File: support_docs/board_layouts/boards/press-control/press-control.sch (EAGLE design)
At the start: 19 parts

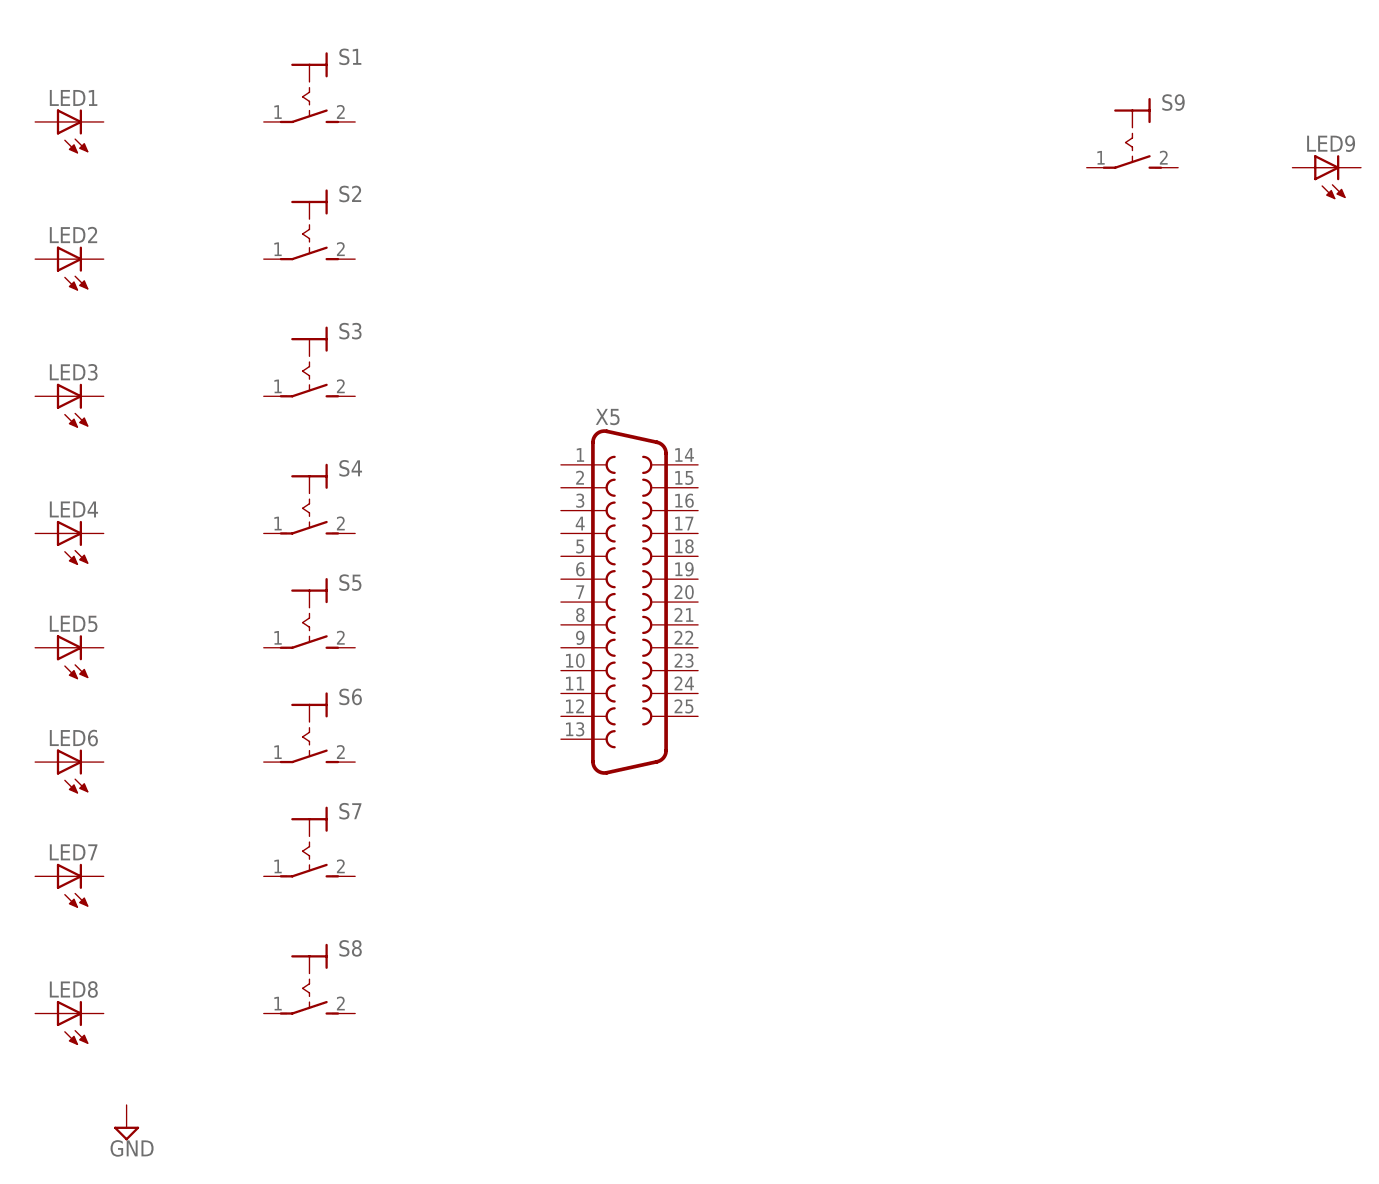
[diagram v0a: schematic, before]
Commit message: new board design
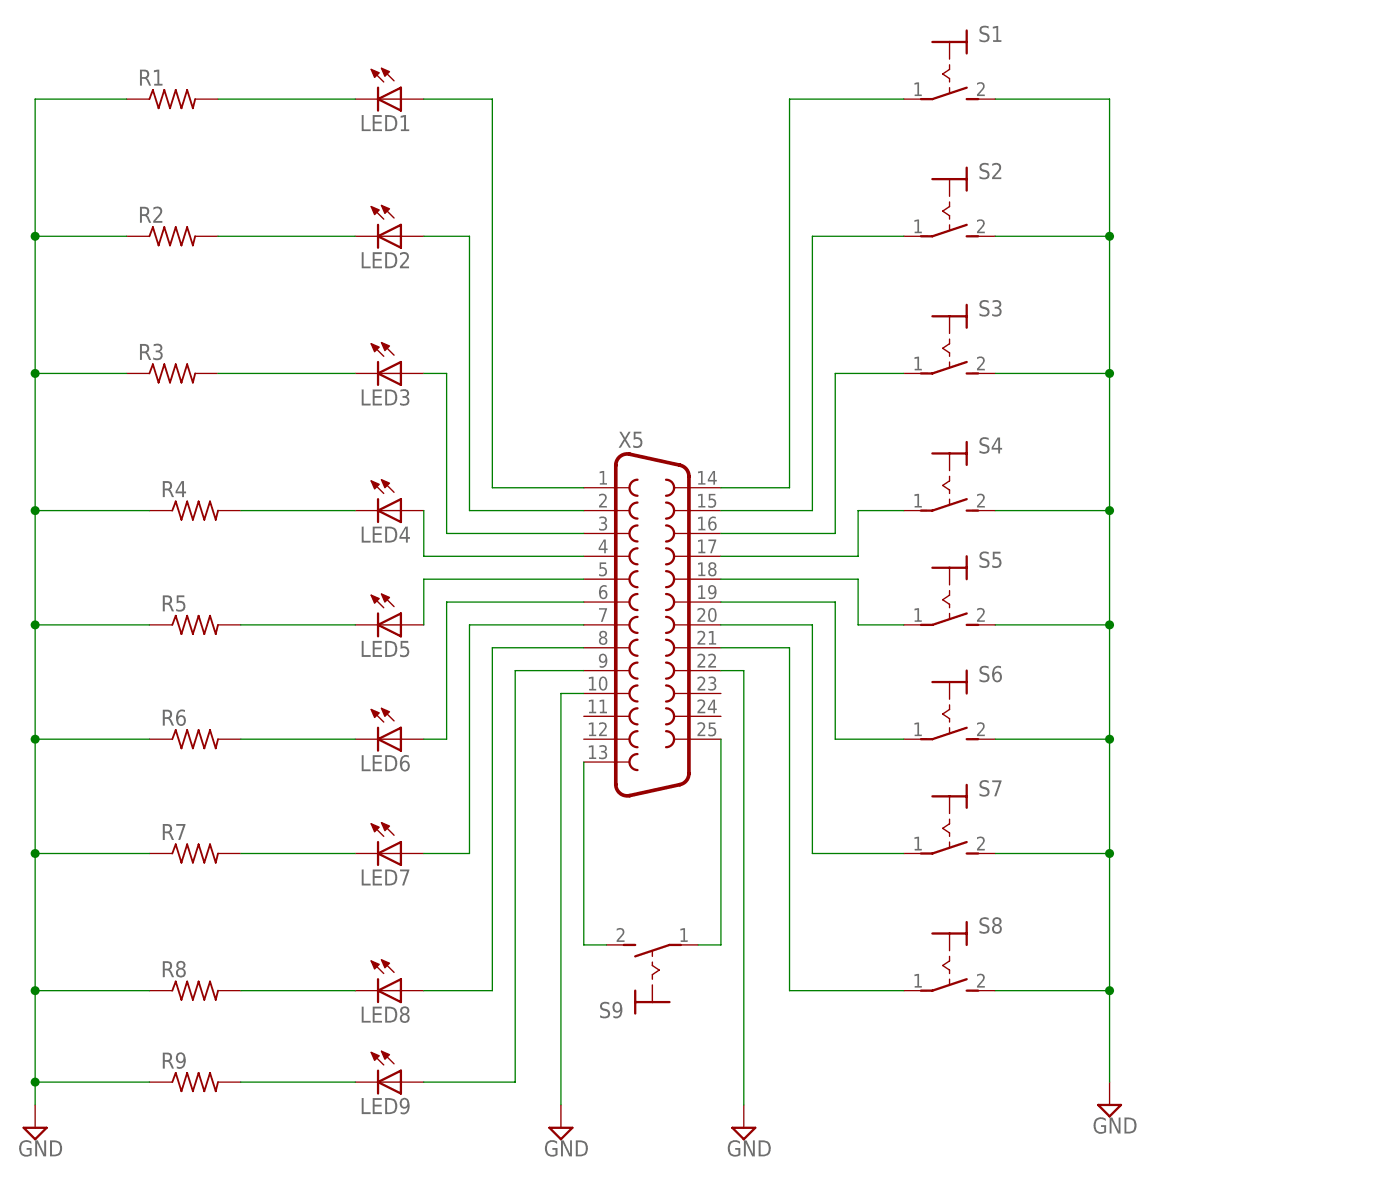
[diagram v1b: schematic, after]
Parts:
- added R1, R2, R3, R4, R5, R6, R7, R8, R9: (no value), resistor:R-US_0207/10
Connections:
- new net GND: R1.1, R2.1, R3.1, R4.1, R5.1, R6.1, R7.1, R8.1, R9.1, S1.S, S2.S, S3.S, S4.S, S5.S, S6.S, S7.S, S8.S, X5.10, X5.22
- new net N$1: LED1.C, R1.2
- new net N$10: LED5.A, X5.5
- new net N$11: LED3.A, X5.3
- new net N$12: LED2.A, X5.2
- new net N$13: LED1.A, X5.1
- new net N$14: LED6.A, X5.6
- new net N$15: LED7.A, X5.7
- new net N$16: LED8.A, X5.8
- new net N$17: S5.P, X5.18
- new net N$18: S4.P, X5.17
- new net N$19: S3.P, X5.16
- new net N$2: LED2.C, R2.2
- new net N$20: S2.P, X5.15
- new net N$21: S1.P, X5.14
- new net N$22: S6.P, X5.19
- new net N$23: S7.P, X5.20
- new net N$24: S8.P, X5.21
- new net N$25: S9.S, X5.13
- new net N$26: S9.P, X5.25
- new net N$27: LED9.A, X5.9
- new net N$28: LED9.C, R9.2
- new net N$3: LED3.C, R3.2
- new net N$4: LED4.C, R4.2
- new net N$5: LED5.C, R5.2
- new net N$6: LED6.C, R6.2
- new net N$7: LED7.C, R7.2
- new net N$8: LED8.C, R8.2
- new net N$9: LED4.A, X5.4
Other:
- moved on the sheet: LED1, LED2, LED3, LED4, LED5, LED6, LED7, LED8, LED9, S1, S2, S3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
